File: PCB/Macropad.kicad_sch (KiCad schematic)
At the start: 27 parts, among them J1 OLED_128x32, SW1 RotaryEncoder_Switch, SW2 RotaryEncoder_Switch, U1 MOUDLE-SEEEDUINO-XIAO

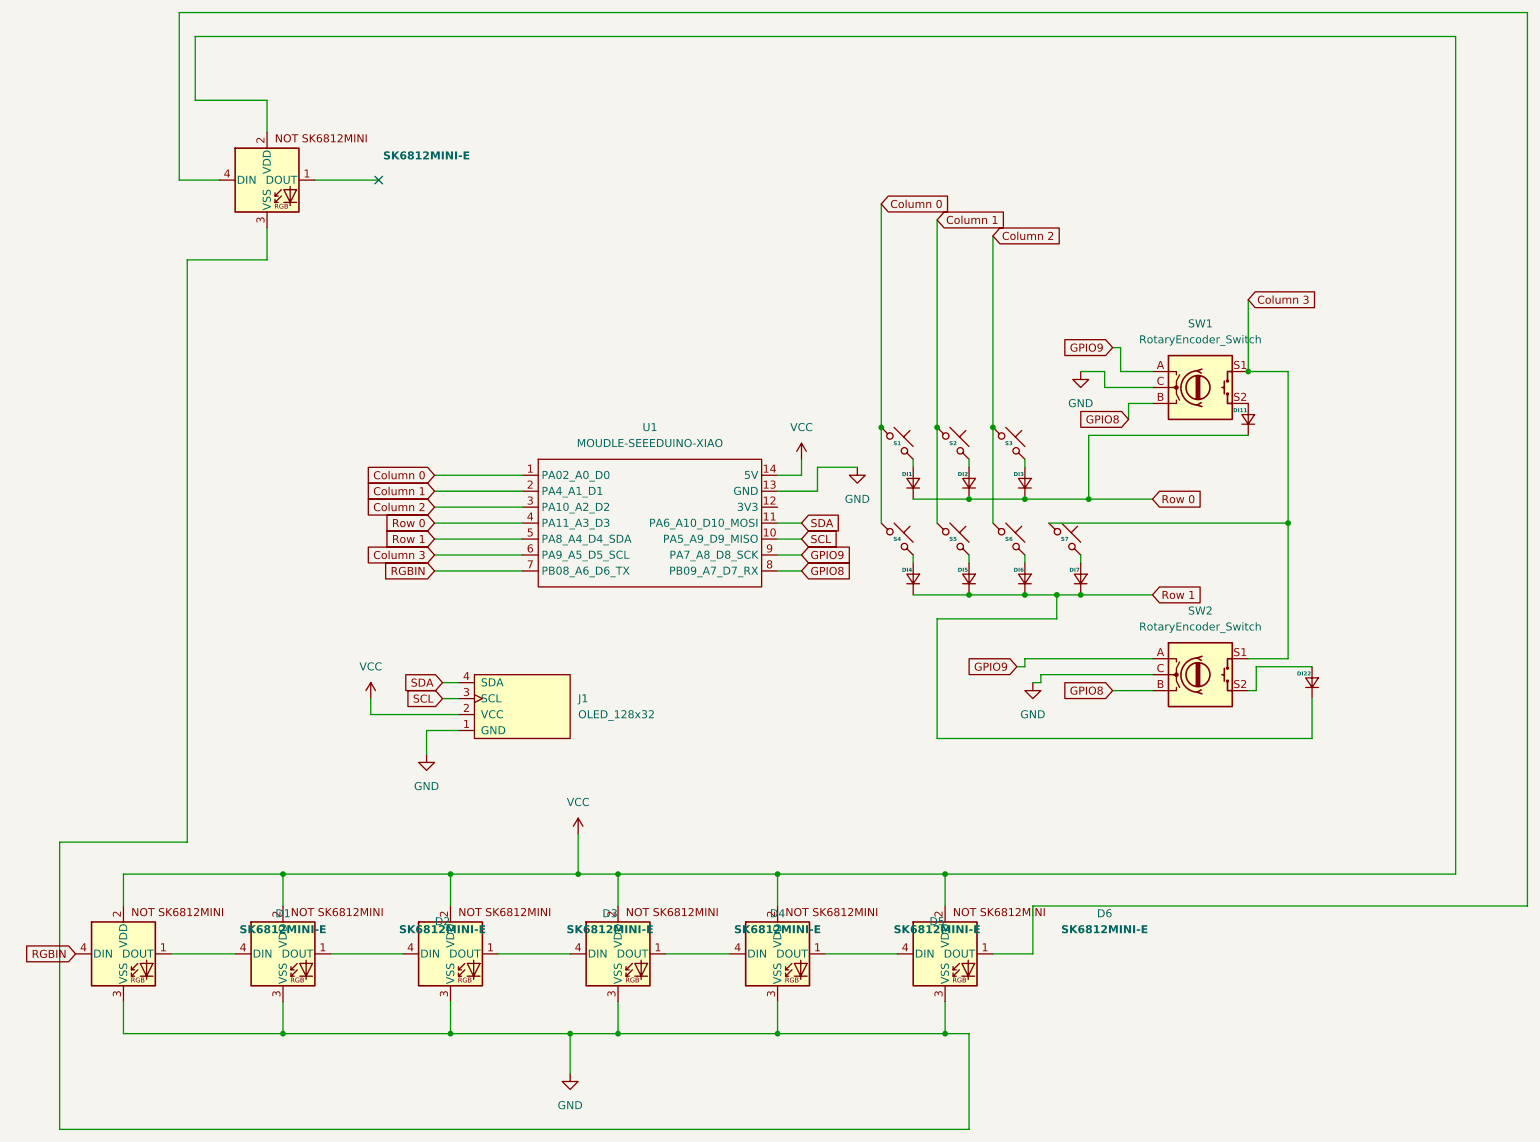
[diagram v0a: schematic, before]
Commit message: replalced exxisting files
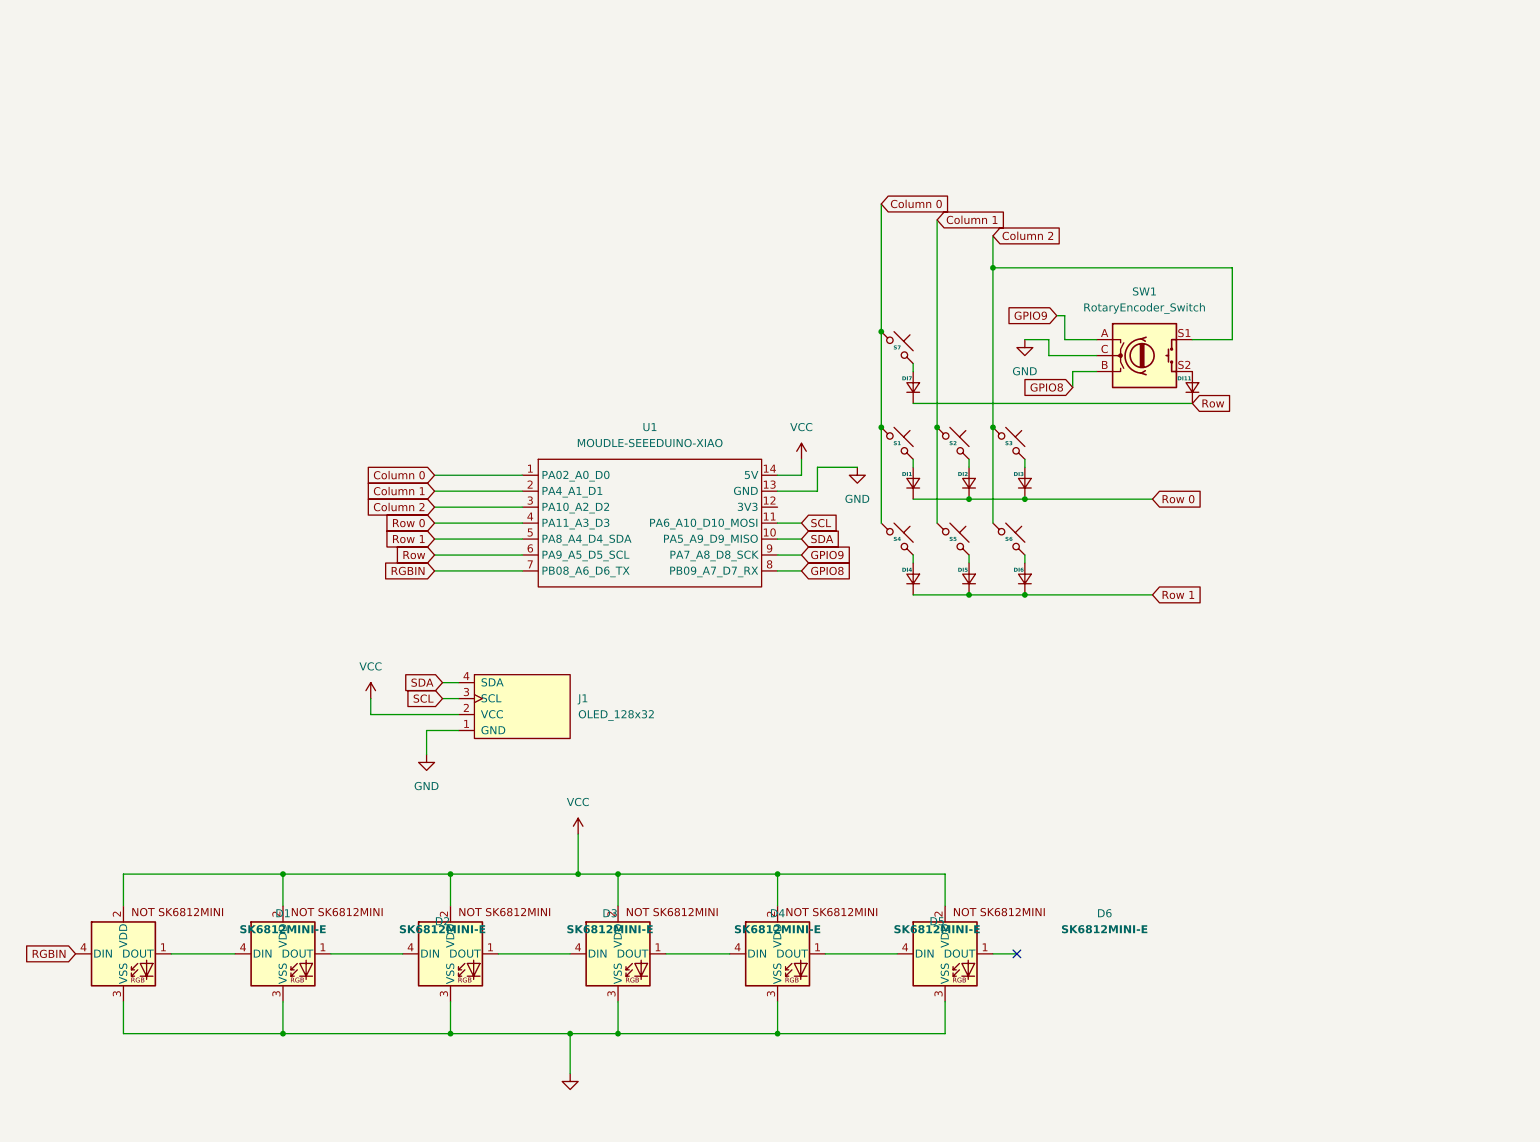
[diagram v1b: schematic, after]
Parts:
- removed D7: SK6812MINI-E, footprints:SK6812MINI-E_fixed, symbol SK6812MINI-E:SK6812MINI-E
- removed DI22: ~, Diode_THT:D_DO-35_SOD27_P10.16mm_Horizontal, symbol ScottoKeebs:Placeholder_Diode
- removed SW2: RotaryEncoder_Switch, Rotary_Encoder:RotaryEncoder_Alps_EC11E-Switch_Vertical_H20mm, symbol Device:RotaryEncoder_Switch
- D1, D2, D3, D4, D5, D6: footprint footprints:SK6812MINI-E_fixed -> ScottoKeebs_Components:LED_SK6812MINI
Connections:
- net Column 0: now also S7.1
- net Column 2: now also SW1.S1
- net Row 0: no longer DI11.1 (K)
- net Row 1: no longer DI7.1 (K)
- net SCL: now also U1.11 (PA6_A10_D10_MOSI); no longer U1.10 (PA5_A9_D9_MISO)
- net SDA: now also U1.10 (PA5_A9_D9_MISO); no longer U1.11 (PA6_A10_D10_MOSI)
- removed net Column 3: S7.1, SW1.S1, U1.6 (PA9_A5_D5_SCL)
- new net Row: DI11.1 (K), DI7.1 (K), U1.6 (PA9_A5_D5_SCL)
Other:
- moved on the sheet: DI11, DI7, S7, SW1
